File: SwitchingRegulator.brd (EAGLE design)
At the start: 92.2 x 74.3 mm, 30 parts, among them J1 APP_2POS_CONFIG5V_HORIZ, J2 APP_2POS_CONFIG5V_HORIZ, J3 APP_2POS_CONFIG5V_HORIZ, Q2 Q_CSD18532KCSPCB, Q3 Q_CSD18532KCSPCB, U1 OKI-78SR-5/1.5-W36HC

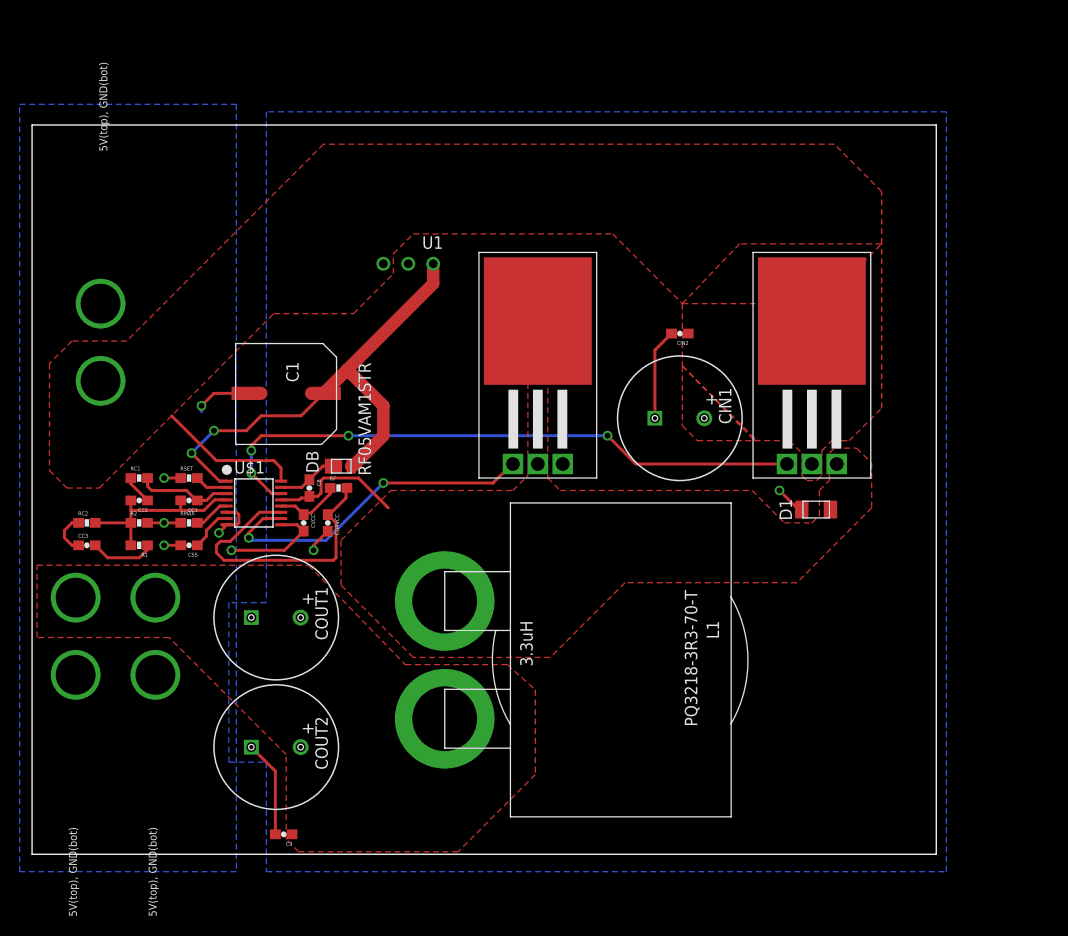
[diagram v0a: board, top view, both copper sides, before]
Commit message: Major rearrangements
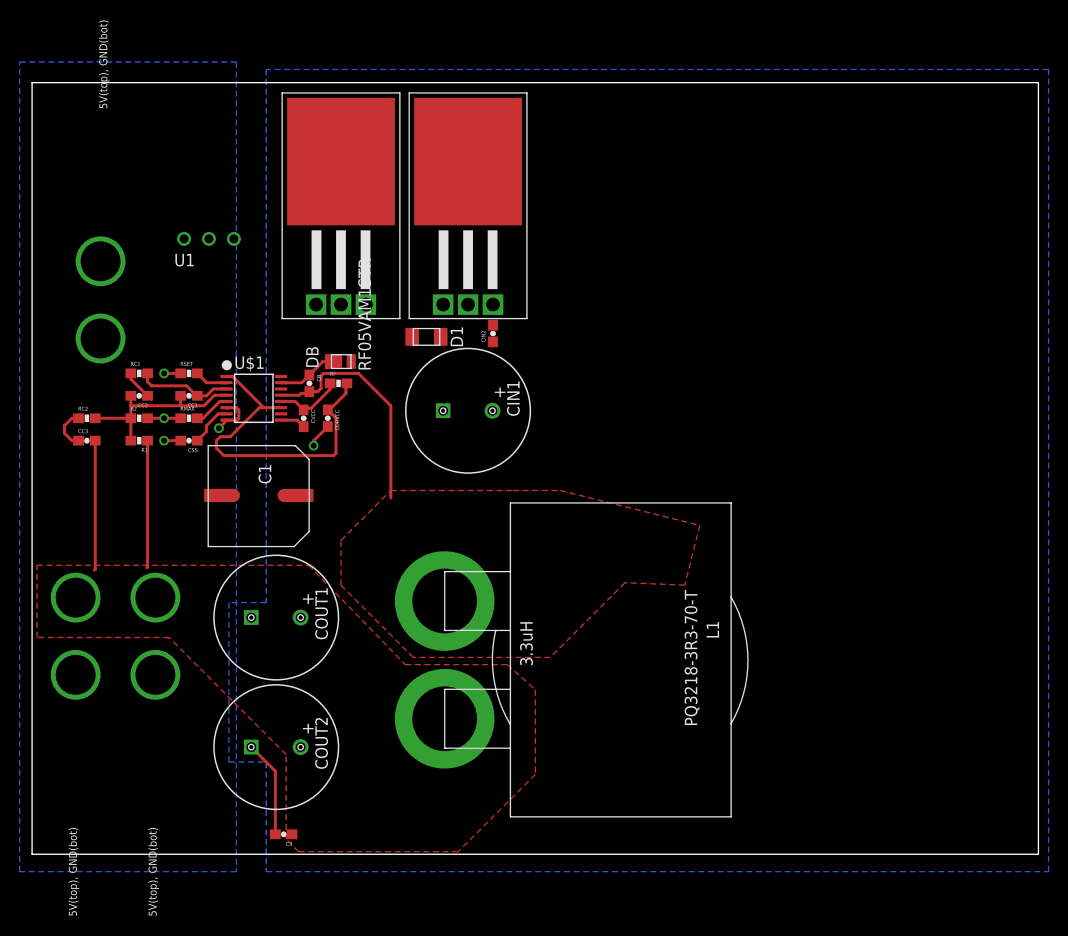
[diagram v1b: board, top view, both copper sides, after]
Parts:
- D1: value RB160MM-30TR -> RBR3MM30ATR
- moved Q2 50.7 mm to (31.5, 70.6)
- moved D1 46.6 mm to (38.9, 53.6), turned to 270 degrees
- moved CIN1 21.6 mm to (44.5, 45.2)
- moved CIN2 19.1 mm to (47.0, 53.1), turned to 90 degrees
- moved Q3 17.7 mm to (44.5, 70.6)
- moved U1 15.5 mm to (20.6, 62.7), turned to 0 degrees
- moved C1 10.8 mm to (23.1, 36.6)
- moved CDRVCC 10.7 mm to (30.1, 44.5)
- moved CVCC 10.7 mm to (27.7, 44.5)
- moved R2 10.7 mm to (10.9, 44.5)
- moved RC2 10.7 mm to (5.59, 44.5)
- moved RMAX 10.7 mm to (16.0, 44.5)
- moved CC3 10.7 mm to (5.59, 42.2)
- moved CSS 10.7 mm to (16.0, 42.2)
- moved R1 10.7 mm to (10.9, 42.2)
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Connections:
- removed net N$12: CC3.2, R1.1
- removed net N$5: C1.+, DB.P$2, U$1.1, U1.3
- net N$15: now also C1.+, DB.P$2, U$1.1, U1.3
- net VOUT12+: now also CC3.2, R1.1
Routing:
- net N$2: track 62.9 -> 0.00 mm, vias 4 -> 0
- net N$5: track 51.4 -> 0.00 mm, vias 2 -> 0
- net N$16: track 34.7 -> 0.00 mm, vias 2 -> 0
- net GND: track 53.4 -> 26.8 mm, vias 8 -> 5
- net VOUT12+: track 0.00 -> 26.2 mm
- net VBATT: track 14.7 -> 0.00 mm
- net N$17: track 13.9 -> 23.6 mm
- net N$12: track 6.63 -> 0.00 mm
- net N$15: track 29.7 -> 34.8 mm
- removed copper zone on layer 1, net VBATT
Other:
- board size 92.2 x 74.3 mm -> 102.6 x 78.7 mm
